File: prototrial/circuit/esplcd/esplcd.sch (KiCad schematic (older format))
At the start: 14 parts, among them U1 ESP-12E

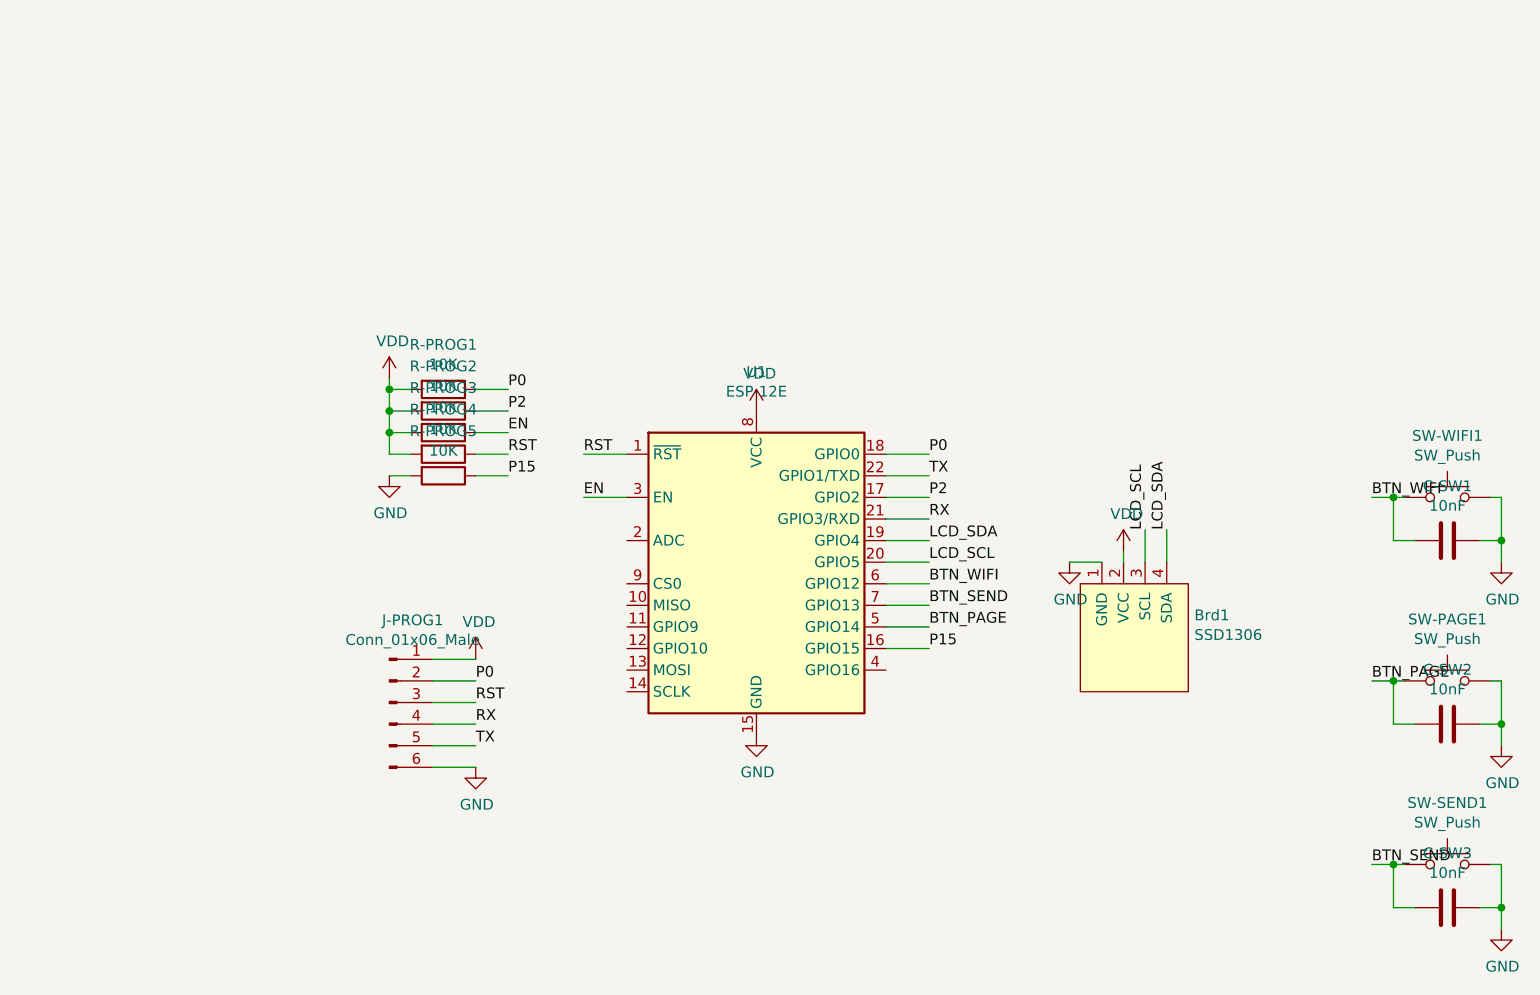
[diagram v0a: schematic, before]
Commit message: paging jalan
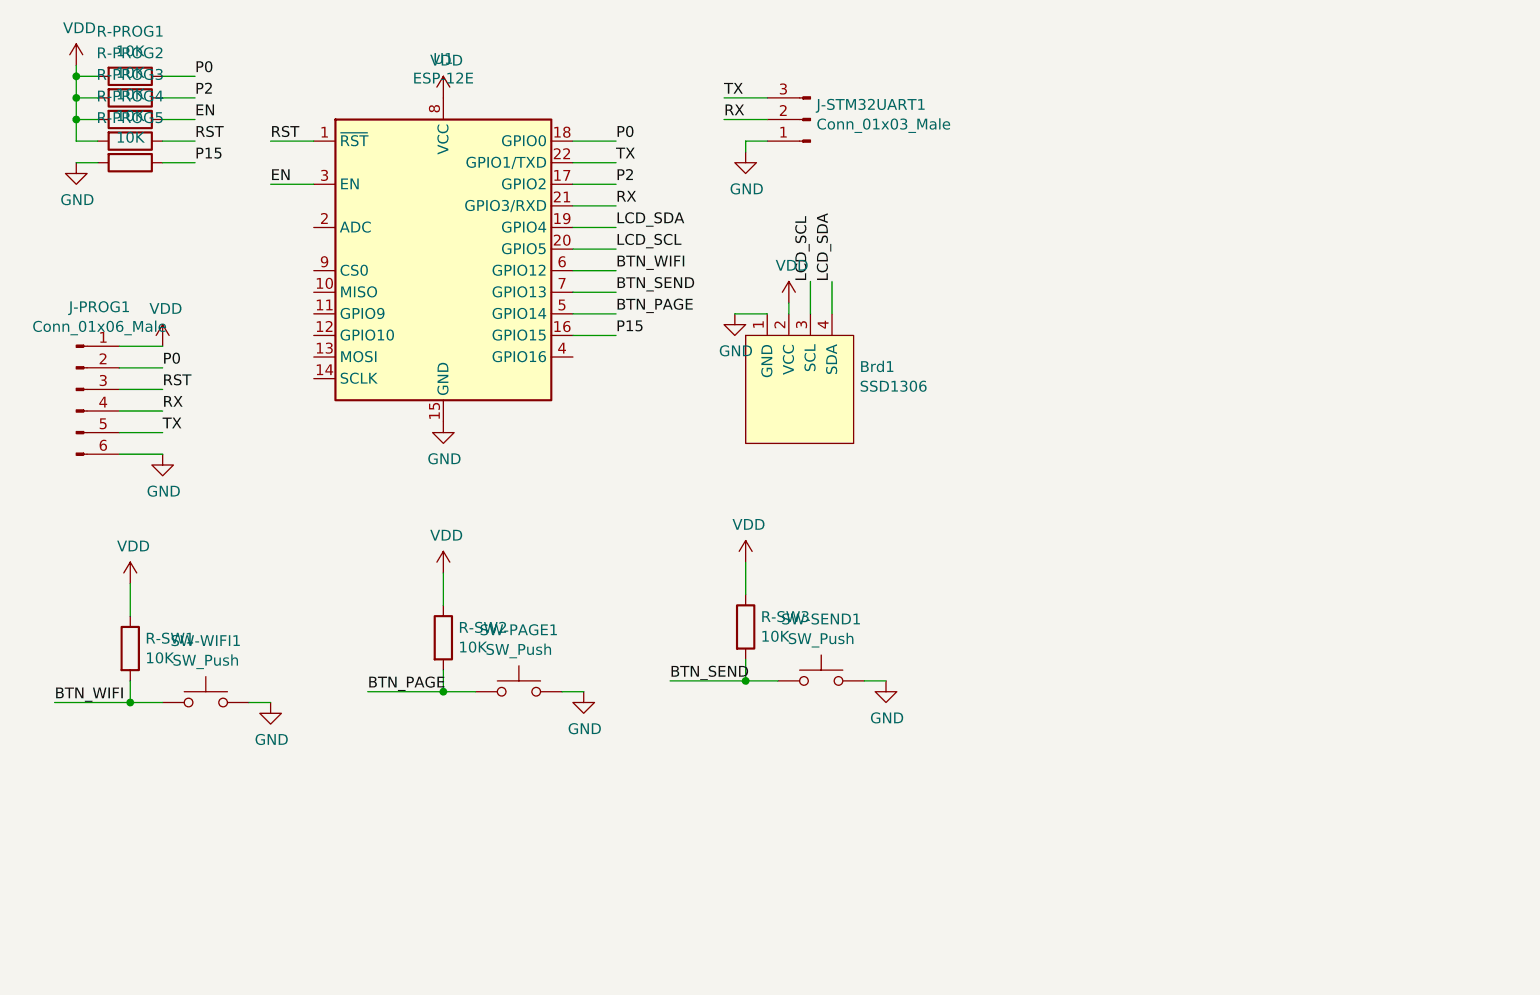
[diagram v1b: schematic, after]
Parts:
- removed C-SW1, C-SW2, C-SW3: 10nF, Capacitor_SMD:C_0201_0603Metric_Pad0.64x0.40mm_HandSolder, symbol Device:C
- added J-STM32UART1: Conn_01x03_Male, Connector_Molex:Molex_KK-254_AE-6410-03A_1x03_P2.54mm_Vertical, symbol Connector:Conn_01x03_Male
- added R-SW1, R-SW2, R-SW3: 10K, Resistor_SMD:R_0805_2012Metric_Pad1.20x1.40mm_HandSolder, symbol Device:R
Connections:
- net BTN_PAGE: now also R-SW2.2
- net BTN_SEND: now also R-SW3.2
- net BTN_WIFI: now also R-SW1.2
- net GND: now also J-STM32UART1.1 (Pin_1)
- net RX: now also J-STM32UART1.2 (Pin_2)
- net TX: now also J-STM32UART1.3 (Pin_3)
- net VDD: now also R-SW1.1, R-SW2.1, R-SW3.1
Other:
- moved on the sheet: Brd1, J-PROG1, R-PROG1, R-PROG2, R-PROG3, R-PROG4, R-PROG5, U1
